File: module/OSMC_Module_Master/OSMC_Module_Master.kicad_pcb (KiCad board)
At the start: 4 copper layers, 34 x 41 mm, 10 parts, among them SW1 SW_Push, SW2 SW_Push, SW3 SW_Push, U1 OSMC Module Board w/pins, U2 24LC02BT-I/OT, U3 PCF8574DWR

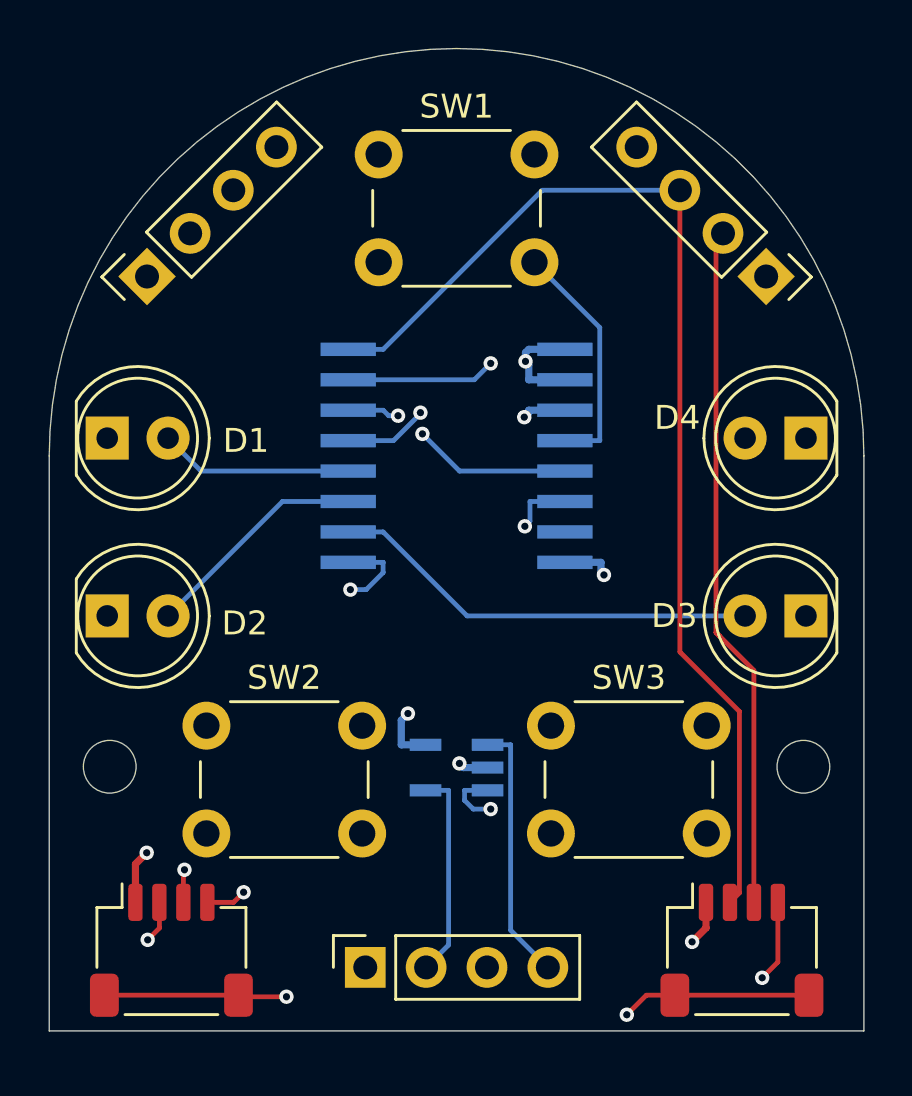
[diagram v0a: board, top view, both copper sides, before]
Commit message: reviewed PCBs
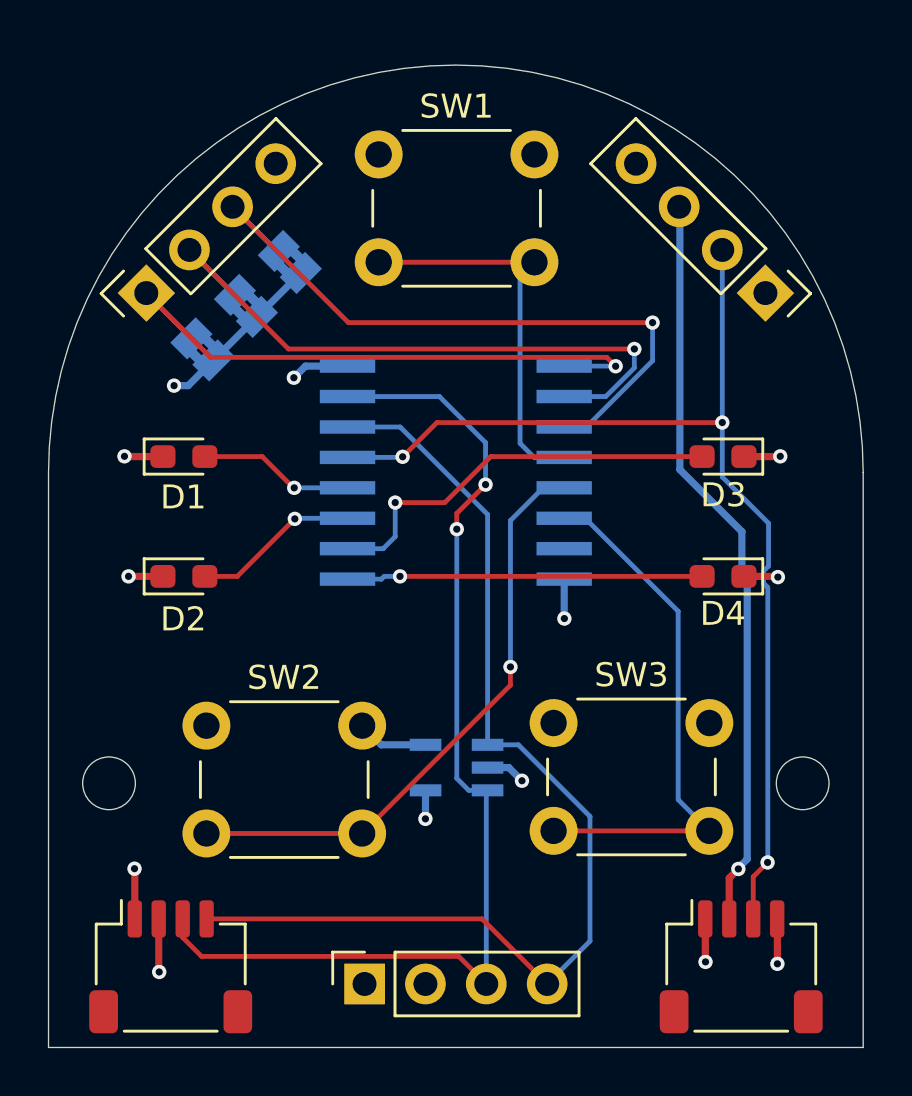
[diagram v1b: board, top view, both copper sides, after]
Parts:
- added J1: SolderJumper_2_Bridged, Jumper:SolderJumper-2_P1.3mm_Bridged2Bar_Pad1.0x1.5mm, B.Cu at (186.4, 71.3)
- added J2: SolderJumper_2_Bridged, Jumper:SolderJumper-2_P1.3mm_Bridged2Bar_Pad1.0x1.5mm, B.Cu at (188.3, 69.5)
- added J3: SolderJumper_2_Bridged, Jumper:SolderJumper-2_P1.3mm_Bridged2Bar_Pad1.0x1.5mm, B.Cu at (190.1, 67.6)
- D1, D2, D3, D4: footprint LED_THT:LED_D5.0mm -> LED_SMD:LED_0603_1608Metric_Pad1.05x0.95mm_HandSolder
- moved D3 7.50 mm to (208.2, 75.8)
- moved D4 6.73 mm to (208.2, 80.8)
- moved D2 3.60 mm to (185.7, 80.8)
- moved D1 3.29 mm to (185.7, 75.8)
- moved U3 0.70 mm to (197.0, 76.4)
- moved U1 0.69 mm to (197.0, 76.4)
- moved SW3 0.16 mm to (201.1, 86.9)
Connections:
- D1 pad 1: GND -> /3v3
- D2 pad 1: GND -> /3v3
- D3 pad 1: GND -> /3v3
- D4 pad 1: GND -> /3v3
- U1 pad 18: unconnected-(U1-A3-Pad18) -> /A2
- U1 pad 19: unconnected-(U1-A2-Pad19) -> /A1
- U1 pad 20: unconnected-(U1-A1-Pad20) -> /A0
- U3 pad 1: GND -> /A0
- U3 pad 16: /5V -> /3v3
- U3 pad 2: GND -> /A1
- U3 pad 3: GND -> /A2
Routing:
- net /3v3: track 71.8 -> 13.7 mm, vias 2 -> 8
- net unconnected-(U1-PadMP)_3: track 30.1 -> 0.00 mm, vias 2 -> 0
- net /A2: track 0.00 -> 28.6 mm, vias 0 -> 1
- net /A1: track 0.00 -> 27.2 mm, vias 0 -> 1
- net /A0: track 0.00 -> 25.7 mm, vias 0 -> 1
- net /5V: track 47.5 -> 31.2 mm, vias 0 -> 1
- net /D4: track 22.6 -> 14.8 mm
- net /B2: track 30.8 -> 24.9 mm
- net /SCL: track 51.3 -> 45.6 mm, vias 2 -> 0
- net /SDA: track 49.3 -> 44.9 mm, vias 3 -> 2
- net /INT: track 48.4 -> 45.4 mm, vias 1 -> 3
- net /D2: track 9.50 -> 6.96 mm, vias 0 -> 1
- net /D1: track 8.09 -> 6.49 mm, vias 0 -> 1
- net GND: track 16.2 -> 17.4 mm, vias 7 -> 5
- net /D3: track 18.0 -> 17.2 mm, vias 0 -> 1
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- added copper zone on In2.Cu, net /3v3
